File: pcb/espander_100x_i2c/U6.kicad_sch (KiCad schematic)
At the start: 0 parts

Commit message: Resync
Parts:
- added J15, J16, J17: DG127A-5.08-06P-14-00AH, DG127A50806P1400AH, symbol 1_tme:DG127A-5.08-06P-14-00AH
- added U6: MCP23017_SP, Package_DIP:DIP-28_W7.62mm, symbol Interface_Expansion:MCP23017_SP
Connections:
- new net +5VD: U6.9 (VDD)
- new net GND: U6.10 (VSS)
- new net SCK: U6.12 (SCK)
- new net SDA: U6.13 (SDA)
- new net U6-GPA0: J16.6, U6.21 (GPA0)
- new net U6-GPA1: J16.5, U6.22 (GPA1)
- new net U6-GPA2: J17.5, U6.23 (GPA2)
- new net U6-GPA3: J17.6, U6.24 (GPA3)
- new net U6-GPA4: J16.1, U6.25 (GPA4)
- new net U6-GPA5: J16.2, U6.26 (GPA5)
- new net U6-GPA6: J16.3, U6.27 (GPA6)
- new net U6-GPA7: J16.4, U6.28 (GPA7)
- new net U6-GPB0: J15.1, U6.1 (GPB0)
- new net U6-GPB1: J15.2, U6.2 (GPB1)
- new net U6-GPB2: J15.3, U6.3 (GPB2)
- new net U6-GPB3: J15.4, U6.4 (GPB3)
- new net U6-GPB4: J15.5, U6.5 (GPB4)
- new net U6-GPB5: J15.6, U6.6 (GPB5)
- new net U6-GPB6: U6.7 (GPB6)
- new net U6-GPB7: U6.8 (GPB7)
- new net U7-GPB4: J17.1
- new net U7-GPB5: J17.2
- new net U7-GPB6: J17.3
- new net U7-GPB7: J17.4

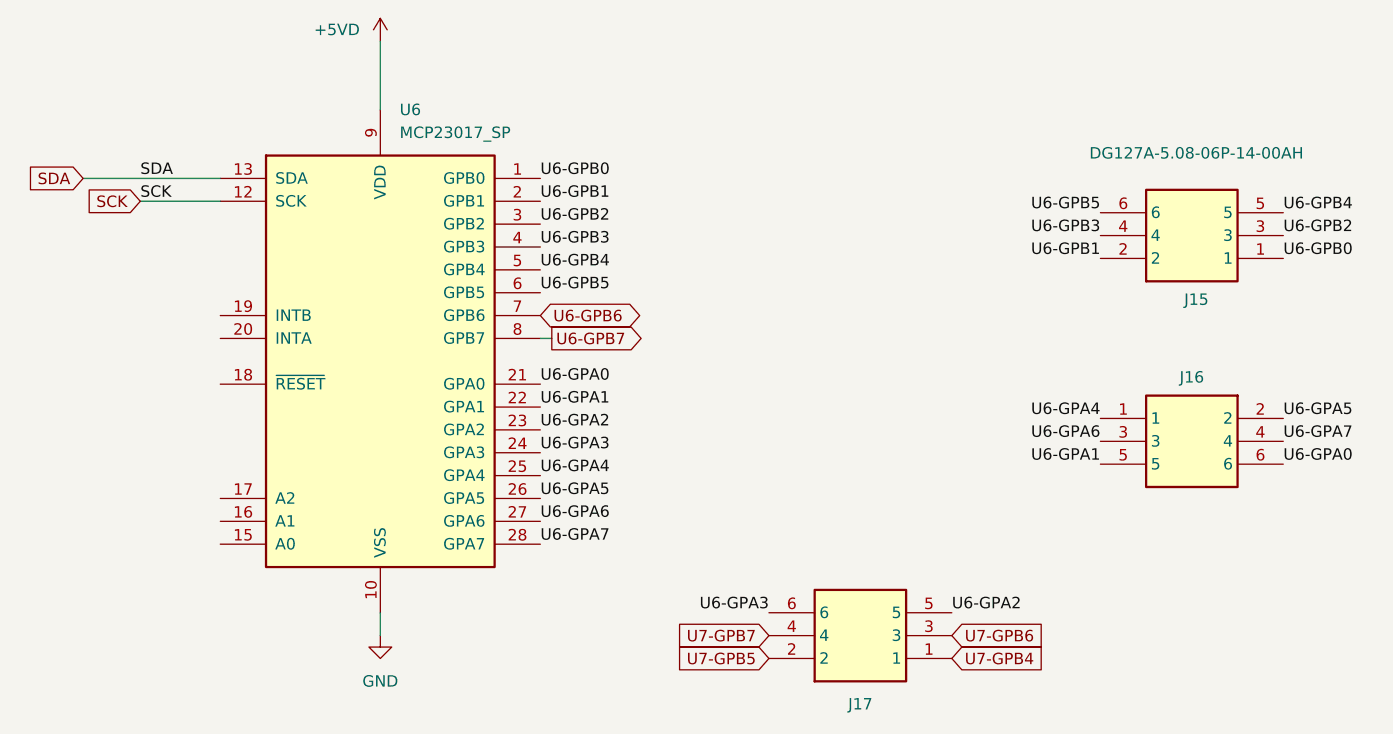
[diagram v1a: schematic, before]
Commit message: resync
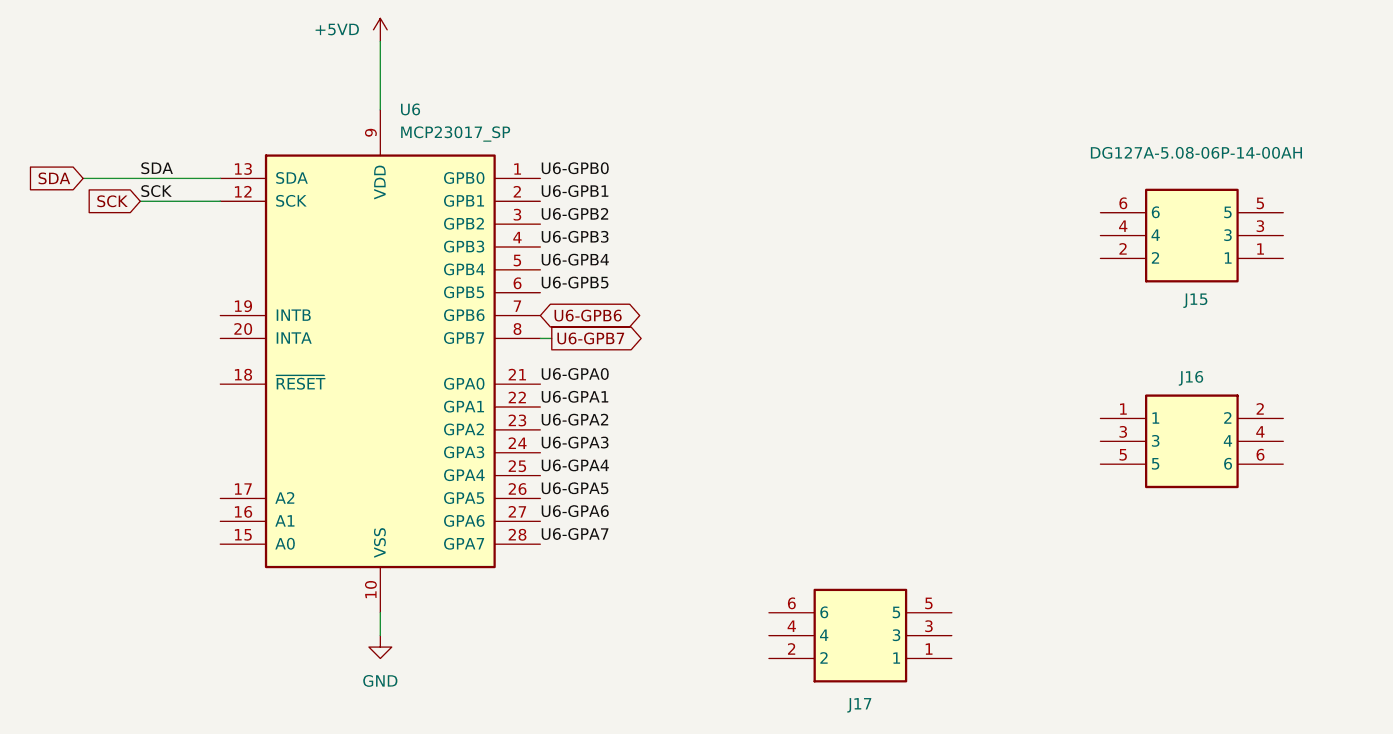
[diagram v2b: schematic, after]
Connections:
- net U6-GPA0: no longer J16.6
- net U6-GPA1: no longer J16.5
- net U6-GPA2: no longer J17.5
- net U6-GPA3: no longer J17.6
- net U6-GPA4: no longer J16.1
- net U6-GPA5: no longer J16.2
- net U6-GPA6: no longer J16.3
- net U6-GPA7: no longer J16.4
- net U6-GPB0: no longer J15.1
- net U6-GPB1: no longer J15.2
- net U6-GPB2: no longer J15.3
- net U6-GPB3: no longer J15.4
- net U6-GPB4: no longer J15.5
- net U6-GPB5: no longer J15.6
- net U7-GPB4: no longer names the net of J17.1
- net U7-GPB5: no longer names the net of J17.2
- net U7-GPB6: no longer names the net of J17.3
- net U7-GPB7: no longer names the net of J17.4
